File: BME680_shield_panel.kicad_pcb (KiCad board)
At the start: 2 copper layers, 73 x 82 mm, 120 parts, among them J101 Conn_01x06, J102 Conn_01x02_Socket, U101 BME680, U102 ESP8266_WeMos_D1_mini, U103 AP7361C-33E, U104 MAX1811

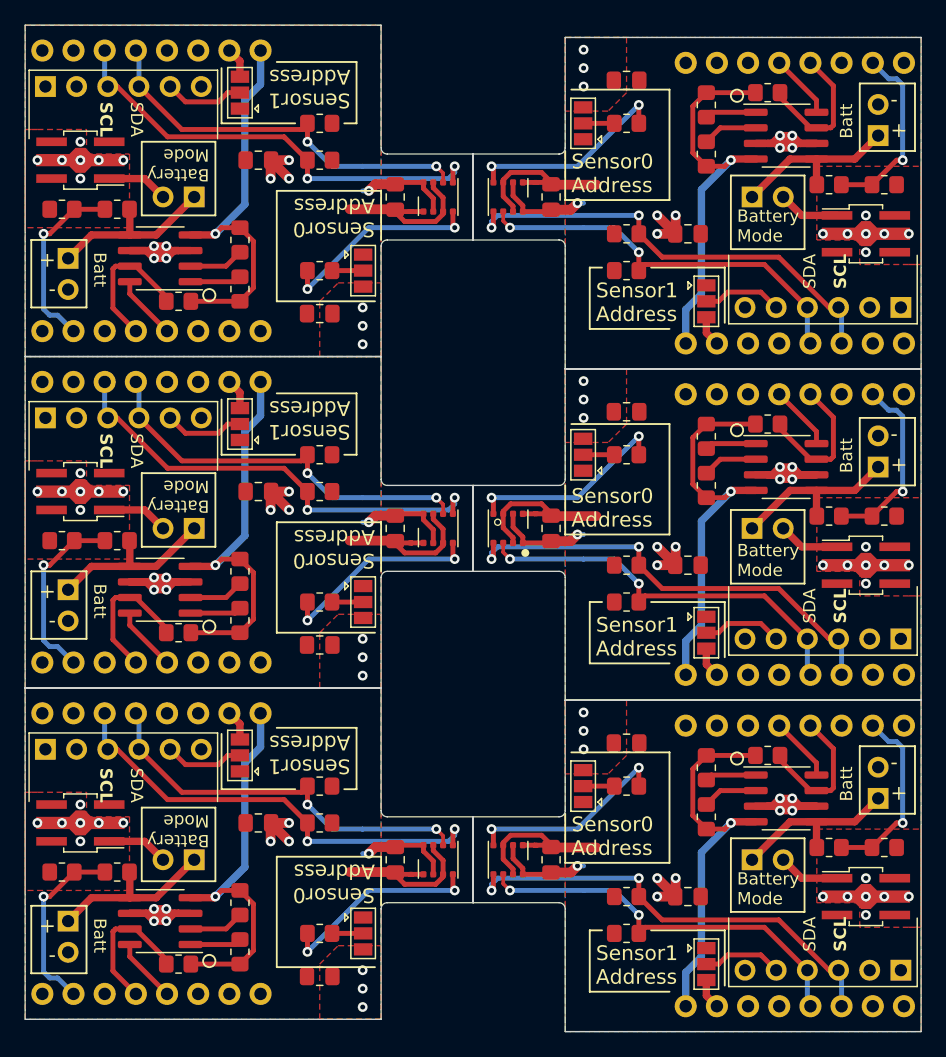
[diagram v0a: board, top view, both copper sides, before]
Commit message: Leiterpaltte aufgebaut
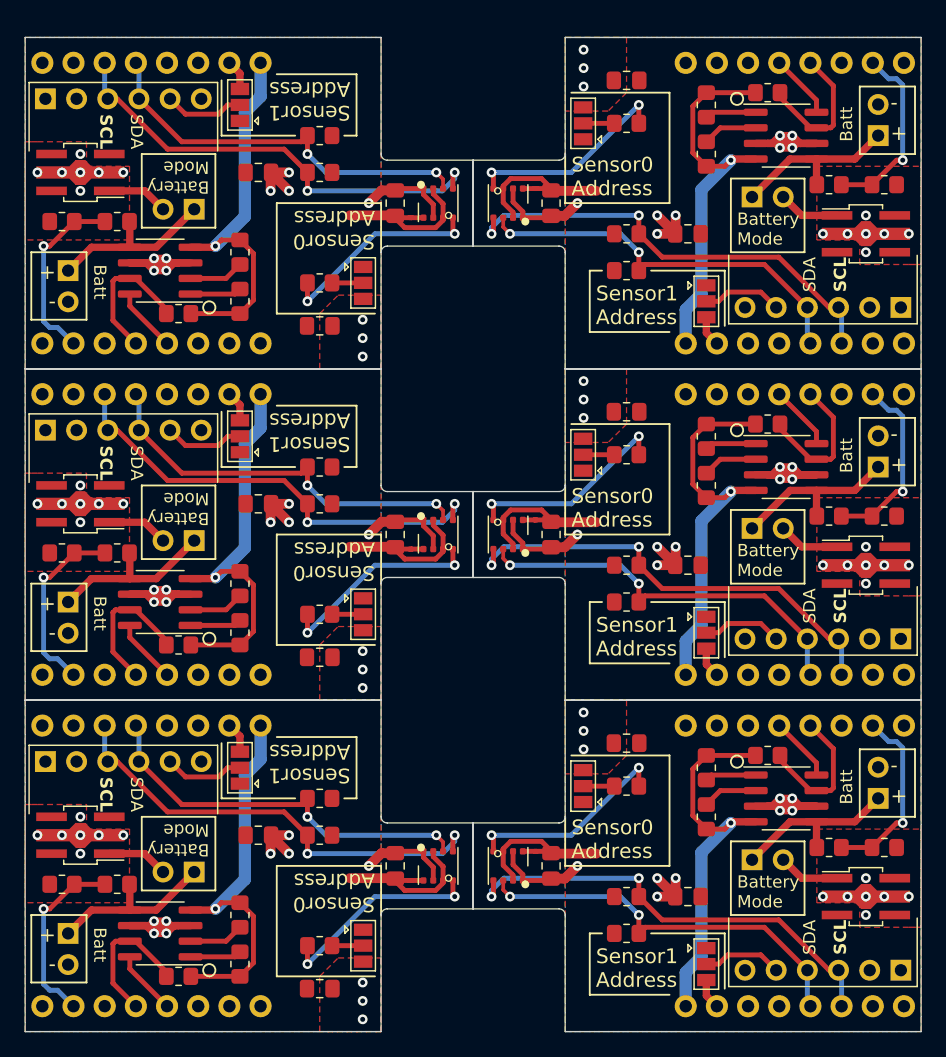
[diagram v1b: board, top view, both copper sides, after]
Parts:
- removed the C101 at (96.8, 41.5)
- removed the C101 at (96.8, 95.5)
- removed the C101 at (84.2, 68.5)
- removed the C101 at (84.2, 41.5)
- removed the C101 at (84.2, 95.5)
- removed the C102 at (78.0, 51.0)
- removed the C102 at (78.0, 105.0)
- removed the C102 at (78.0, 78.0)
- removed the C103 at (73.0, 92.5)
- removed the C103 at (73.0, 38.5)
- removed the C103 at (73.0, 65.5)
- removed the J101 at (55.6, 59.5)
- removed the J101 at (55.6, 32.5)
- removed the J101 at (55.6, 86.5)
- removed the J102 at (57.5, 73.5)
- removed the J102 at (57.5, 46.5)
- removed the J102 at (57.5, 100.5)
- removed the JP101 at (71.5, 87.0)
- removed the JP101 at (71.5, 33.0)
- removed the JP101 at (71.5, 60.0)
- removed the JP102 at (81.5, 101.5)
- removed the JP102 at (81.5, 47.5)
- removed the JP102 at (81.5, 74.5)
- removed the JP103 at (67.8, 41.5)
- removed the JP103 at (67.8, 95.5)
- removed the JP103 at (67.8, 68.5)
- removed the R101 at (78.0, 101.5)
- removed the R101 at (78.0, 74.5)
- removed the R101 at (78.0, 47.5)
- removed the R102 at (78.0, 92.5)
- removed the R102 at (78.0, 65.5)
- removed the R102 at (78.0, 38.5)
- removed the R103 at (78.0, 89.5)
- removed the R103 at (78.0, 35.5)
- removed the R103 at (78.0, 62.5)
- removed the R104 at (61.5, 42.5)
- removed the R104 at (61.5, 96.5)
- removed the R104 at (61.5, 69.5)
- removed the R105 at (57.0, 69.5)
- removed the R105 at (57.0, 96.5)
- removed the R105 at (57.0, 42.5)
- removed the R106 at (71.5, 45.0)
- removed the R106 at (71.5, 72.0)
- removed the R106 at (71.5, 99.0)
- removed the R107 at (71.5, 76.0)
- removed the R107 at (71.5, 49.0)
- removed the R107 at (71.5, 103.0)
- removed the R108 at (66.5, 77.0)
- removed the R108 at (66.5, 104.0)
- removed the R108 at (66.5, 50.0)
- removed the U101 at (93.3, 95.5)
- removed the U101 at (87.7, 68.5)
- removed the U101 at (87.7, 41.5)
- removed the U101 at (87.7, 95.5)
- removed the U101 at (93.3, 41.5)
- removed the U102 at (64.3, 95.0)
- removed the U102 at (64.3, 68.0)
- removed the U102 at (64.3, 41.0)
- removed the U103 at (58.5, 92.5)
- removed the U103 at (58.5, 65.5)
- removed the U103 at (58.5, 38.5)
- removed the U104 at (65.0, 46.5)
- removed the U104 at (65.0, 100.5)
- removed the U104 at (65.0, 73.5)
- added C101: 100n, Capacitor_SMD:C_0805_2012Metric_Pad1.18x1.45mm_HandSolder, F.Cu at (84.2, 96.0)
- added C101: 100n, Capacitor_SMD:C_0805_2012Metric_Pad1.18x1.45mm_HandSolder, F.Cu at (84.2, 42.0)
- added C101: 100n, Capacitor_SMD:C_0805_2012Metric_Pad1.18x1.45mm_HandSolder, F.Cu at (96.8, 96.0)
- added C101: 100n, Capacitor_SMD:C_0805_2012Metric_Pad1.18x1.45mm_HandSolder, F.Cu at (84.2, 69.0)
- added C101: 100n, Capacitor_SMD:C_0805_2012Metric_Pad1.18x1.45mm_HandSolder, F.Cu at (96.8, 42.0)
- added C102: 10µ, Capacitor_SMD:C_0805_2012Metric_Pad1.18x1.45mm_HandSolder, F.Cu at (78.0, 79.0)
- added C102: 10µ, Capacitor_SMD:C_0805_2012Metric_Pad1.18x1.45mm_HandSolder, F.Cu at (78.0, 52.0)
- added C102: 10µ, Capacitor_SMD:C_0805_2012Metric_Pad1.18x1.45mm_HandSolder, F.Cu at (78.0, 106.0)
- added C103: 10µ, Capacitor_SMD:C_0805_2012Metric_Pad1.18x1.45mm_HandSolder, F.Cu at (73.0, 39.5)
- added C103: 10µ, Capacitor_SMD:C_0805_2012Metric_Pad1.18x1.45mm_HandSolder, F.Cu at (73.0, 93.5)
- added C103: 10µ, Capacitor_SMD:C_0805_2012Metric_Pad1.18x1.45mm_HandSolder, F.Cu at (73.0, 66.5)
- added J101: Conn_01x06, Connector_PinHeader_2.54mm:PinHeader_1x06_P2.54mm_Vertical, F.Cu at (55.6, 87.5)
- added J101: Conn_01x06, Connector_PinHeader_2.54mm:PinHeader_1x06_P2.54mm_Vertical, F.Cu at (55.6, 33.5)
- added J101: Conn_01x06, Connector_PinHeader_2.54mm:PinHeader_1x06_P2.54mm_Vertical, F.Cu at (55.6, 60.5)
- added J102: Conn_01x02_Socket, Connector_PinHeader_2.54mm:PinHeader_1x02_P2.54mm_Vertical, F.Cu at (57.5, 47.5)
- added J102: Conn_01x02_Socket, Connector_PinHeader_2.54mm:PinHeader_1x02_P2.54mm_Vertical, F.Cu at (57.5, 101.5)
- added J102: Conn_01x02_Socket, Connector_PinHeader_2.54mm:PinHeader_1x02_P2.54mm_Vertical, F.Cu at (57.5, 74.5)
- added JP101: Jumper_3_Open, Jumper:SolderJumper-3_P1.3mm_Open_Pad1.0x1.5mm, F.Cu at (71.5, 61.0)
- added JP101: Jumper_3_Open, Jumper:SolderJumper-3_P1.3mm_Open_Pad1.0x1.5mm, F.Cu at (71.5, 34.0)
- added JP101: Jumper_3_Open, Jumper:SolderJumper-3_P1.3mm_Open_Pad1.0x1.5mm, F.Cu at (71.5, 88.0)
- added JP102: Jumper_3_Open, Jumper:SolderJumper-3_P1.3mm_Open_Pad1.0x1.5mm, F.Cu at (81.5, 75.5)
- added JP102: Jumper_3_Open, Jumper:SolderJumper-3_P1.3mm_Open_Pad1.0x1.5mm, F.Cu at (81.5, 48.5)
- added JP102: Jumper_3_Open, Jumper:SolderJumper-3_P1.3mm_Open_Pad1.0x1.5mm, F.Cu at (81.5, 102.5)
- added JP103: Jumper_2_Bridged, Connector_PinHeader_2.54mm:PinHeader_1x02_P2.54mm_Vertical, F.Cu at (67.8, 42.5)
- added JP103: Jumper_2_Bridged, Connector_PinHeader_2.54mm:PinHeader_1x02_P2.54mm_Vertical, F.Cu at (67.8, 96.5)
- added JP103: Jumper_2_Bridged, Connector_PinHeader_2.54mm:PinHeader_1x02_P2.54mm_Vertical, F.Cu at (67.8, 69.5)
- added R101: 4k7, Resistor_SMD:R_0805_2012Metric_Pad1.20x1.40mm_HandSolder, F.Cu at (78.0, 102.5)
- added R101: 4k7, Resistor_SMD:R_0805_2012Metric_Pad1.20x1.40mm_HandSolder, F.Cu at (78.0, 75.5)
- added R101: 4k7, Resistor_SMD:R_0805_2012Metric_Pad1.20x1.40mm_HandSolder, F.Cu at (78.0, 48.5)
- added R102: 4k7, Resistor_SMD:R_0805_2012Metric_Pad1.20x1.40mm_HandSolder, F.Cu at (78.0, 39.5)
- added R102: 4k7, Resistor_SMD:R_0805_2012Metric_Pad1.20x1.40mm_HandSolder, F.Cu at (78.0, 93.5)
- added R102: 4k7, Resistor_SMD:R_0805_2012Metric_Pad1.20x1.40mm_HandSolder, F.Cu at (78.0, 66.5)
- added R103: 4k7, Resistor_SMD:R_0805_2012Metric_Pad1.20x1.40mm_HandSolder, F.Cu at (78.0, 63.5)
- added R103: 4k7, Resistor_SMD:R_0805_2012Metric_Pad1.20x1.40mm_HandSolder, F.Cu at (78.0, 36.5)
- added R103: 4k7, Resistor_SMD:R_0805_2012Metric_Pad1.20x1.40mm_HandSolder, F.Cu at (78.0, 90.5)
- added R104: R, Resistor_SMD:R_0805_2012Metric_Pad1.20x1.40mm_HandSolder, F.Cu at (61.5, 70.5)
- added R104: R, Resistor_SMD:R_0805_2012Metric_Pad1.20x1.40mm_HandSolder, F.Cu at (61.5, 43.5)
- added R104: R, Resistor_SMD:R_0805_2012Metric_Pad1.20x1.40mm_HandSolder, F.Cu at (61.5, 97.5)
- added R105: R, Resistor_SMD:R_0805_2012Metric_Pad1.20x1.40mm_HandSolder, F.Cu at (57.0, 70.5)
- added R105: R, Resistor_SMD:R_0805_2012Metric_Pad1.20x1.40mm_HandSolder, F.Cu at (57.0, 97.5)
- added R105: R, Resistor_SMD:R_0805_2012Metric_Pad1.20x1.40mm_HandSolder, F.Cu at (57.0, 43.5)
- added R106: 100k, Resistor_SMD:R_0805_2012Metric_Pad1.20x1.40mm_HandSolder, F.Cu at (71.5, 46.0)
- added R106: 100k, Resistor_SMD:R_0805_2012Metric_Pad1.20x1.40mm_HandSolder, F.Cu at (71.5, 100.0)
- added R106: 100k, Resistor_SMD:R_0805_2012Metric_Pad1.20x1.40mm_HandSolder, F.Cu at (71.5, 73.0)
- added R107: 100k, Resistor_SMD:R_0805_2012Metric_Pad1.20x1.40mm_HandSolder, F.Cu at (71.5, 104.0)
- added R107: 100k, Resistor_SMD:R_0805_2012Metric_Pad1.20x1.40mm_HandSolder, F.Cu at (71.5, 77.0)
- added R107: 100k, Resistor_SMD:R_0805_2012Metric_Pad1.20x1.40mm_HandSolder, F.Cu at (71.5, 50.0)
- added R108: 100k, Resistor_SMD:R_0805_2012Metric_Pad1.20x1.40mm_HandSolder, F.Cu at (66.5, 78.0)
- added R108: 100k, Resistor_SMD:R_0805_2012Metric_Pad1.20x1.40mm_HandSolder, F.Cu at (66.5, 51.0)
- added R108: 100k, Resistor_SMD:R_0805_2012Metric_Pad1.20x1.40mm_HandSolder, F.Cu at (66.5, 105.0)
- added U101: BME680, Package_LGA:Bosch_LGA-8_3x3mm_P0.8mm_ClockwisePinNumbering, F.Cu at (93.3, 96.0)
- added U101: BME680, Package_LGA:Bosch_LGA-8_3x3mm_P0.8mm_ClockwisePinNumbering, F.Cu at (93.3, 42.0)
- added U101: BME680, Package_LGA:Bosch_LGA-8_3x3mm_P0.8mm_ClockwisePinNumbering, F.Cu at (87.7, 69.0)
- added U101: BME680, Package_LGA:Bosch_LGA-8_3x3mm_P0.8mm_ClockwisePinNumbering, F.Cu at (87.7, 96.0)
- added U101: BME680, Package_LGA:Bosch_LGA-8_3x3mm_P0.8mm_ClockwisePinNumbering, F.Cu at (87.7, 42.0)
- added U102: ESP8266_WeMos_D1_mini, ESP8266:wemos-d1-mini-connectors-only, F.Cu at (64.3, 96.0)
- added U102: ESP8266_WeMos_D1_mini, ESP8266:wemos-d1-mini-connectors-only, F.Cu at (64.3, 69.0)
- added U102: ESP8266_WeMos_D1_mini, ESP8266:wemos-d1-mini-connectors-only, F.Cu at (64.3, 42.0)
- added U103: AP7361C-33E, Package_TO_SOT_SMD:SOT-89-5_Handsoldering, F.Cu at (58.5, 93.5)
- added U103: AP7361C-33E, Package_TO_SOT_SMD:SOT-89-5_Handsoldering, F.Cu at (58.5, 39.5)
- added U103: AP7361C-33E, Package_TO_SOT_SMD:SOT-89-5_Handsoldering, F.Cu at (58.5, 66.5)
- added U104: MAX1811, Package_SO:SOIC-8_3.9x4.9mm_P1.27mm, F.Cu at (65.0, 47.5)
- added U104: MAX1811, Package_SO:SOIC-8_3.9x4.9mm_P1.27mm, F.Cu at (65.0, 101.5)
- added U104: MAX1811, Package_SO:SOIC-8_3.9x4.9mm_P1.27mm, F.Cu at (65.0, 74.5)
- moved C101 0.50 mm to (96.8, 69.0)
- moved U101 0.50 mm to (93.3, 69.0)
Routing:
- net GND: track 172.1 -> 170.3 mm
- net Net-(U101-SDO): track 101.7 -> 102.9 mm
- net Net-(J101-Pin_4): track 197.2 -> 196.0 mm
- net Net-(J101-Pin_3): track 224.2 -> 225.5 mm
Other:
- board size 73 x 82 mm -> 73 x 81 mm
